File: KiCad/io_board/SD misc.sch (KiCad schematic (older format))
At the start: 5 parts, among them U10 74HC367, U11 74HC367, U14 74HCT32, U8 74HC245, U9 62256

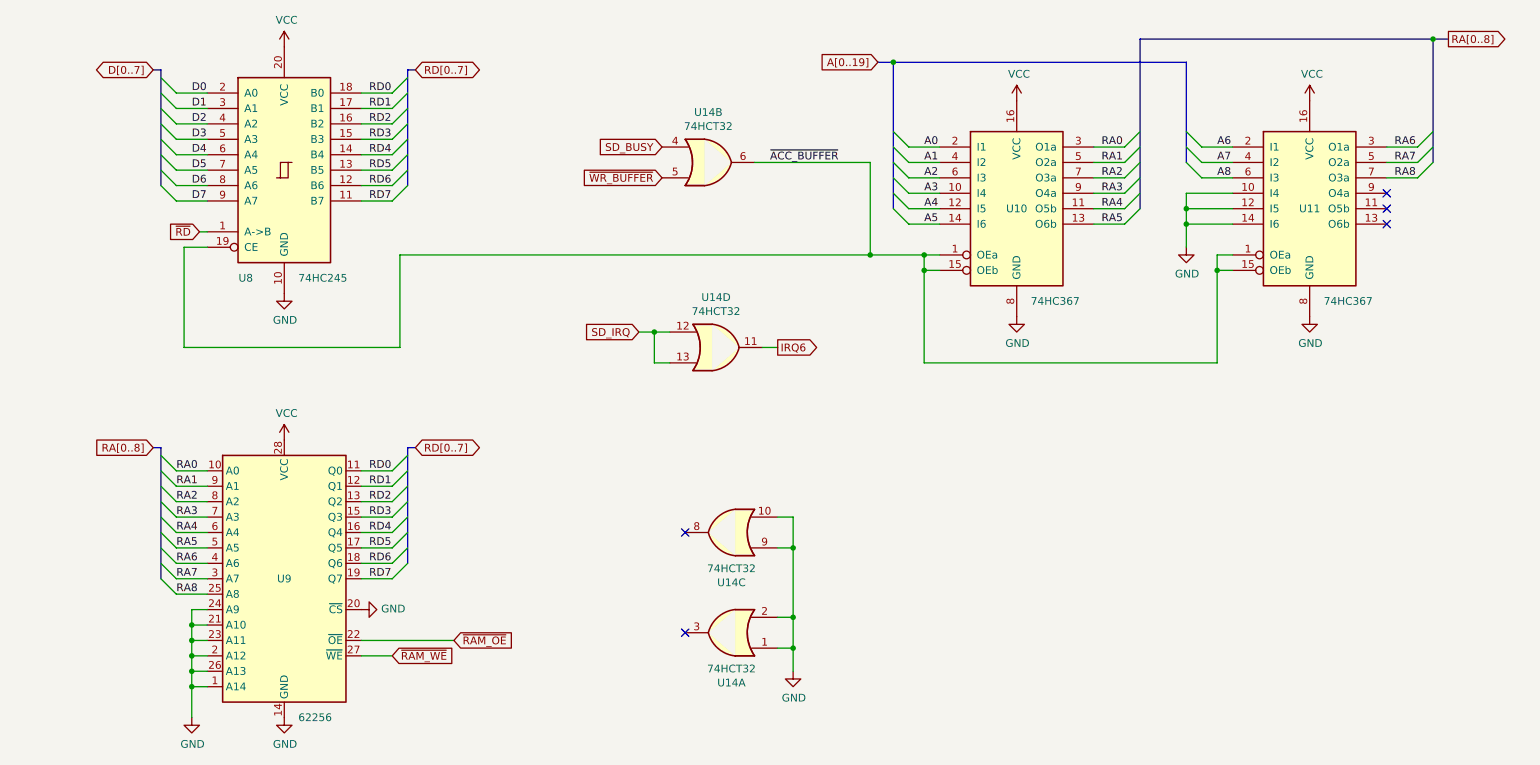
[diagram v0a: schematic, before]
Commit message: Updated I/O board
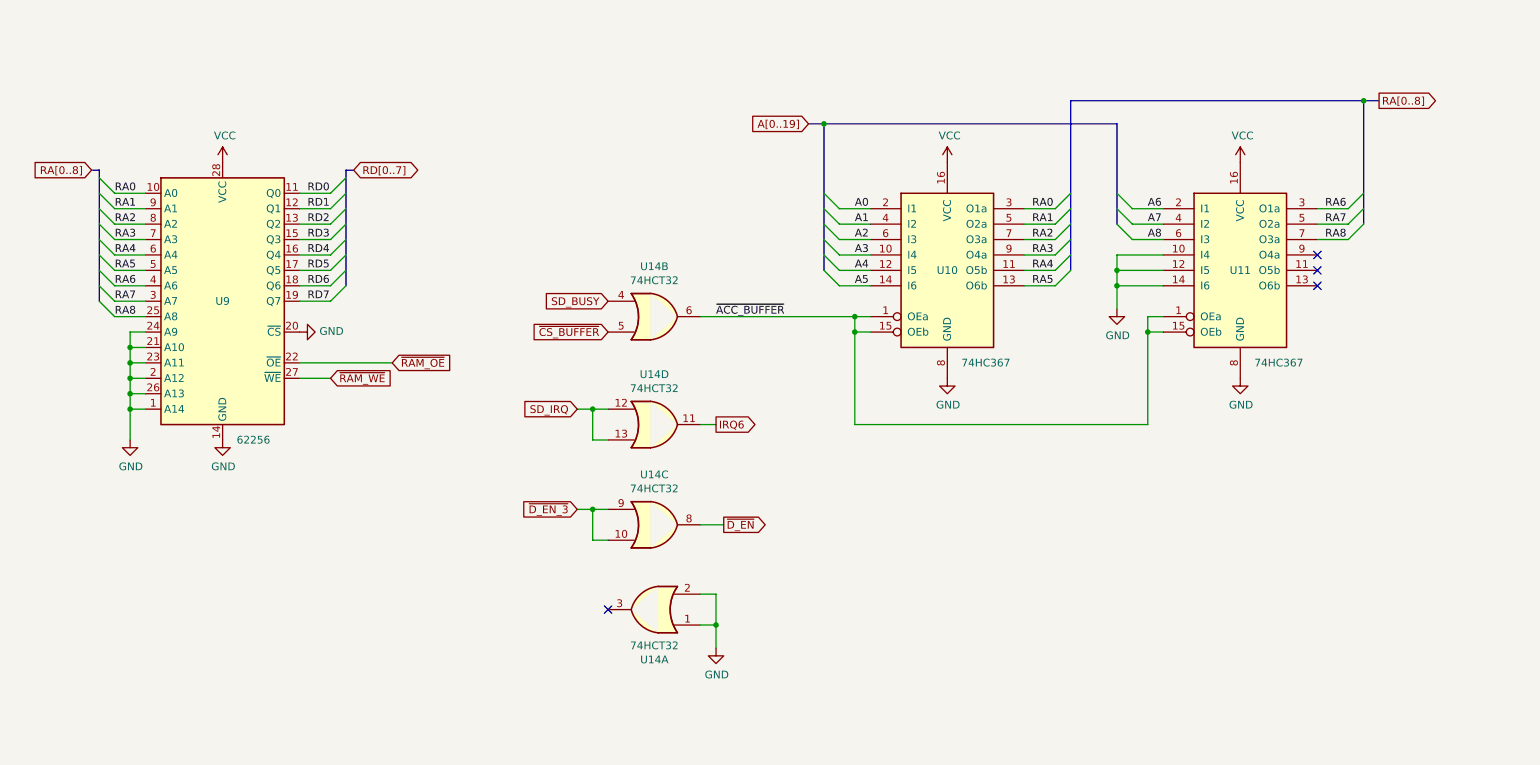
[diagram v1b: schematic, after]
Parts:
- removed U8: 74HC245, Package_SO:SOIC-20W_7.5x12.8mm_P1.27mm, symbol 74xx:74HC245
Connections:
- net GND: no longer U14.10, U14.9
- net ~D_EN: now reaches U14.8
- net ~WR_BUFFER renamed ~CS_BUFFER
- new net ~D_EN_3: U14.10, U14.9
- no-connect marks 5 -> 4
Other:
- moved on the sheet: U10, U11, U14A, U14B, U14C, U14D, U9
